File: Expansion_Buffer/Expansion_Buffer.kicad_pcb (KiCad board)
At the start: 2 copper layers, 23 x 62 mm, 18 parts, among them J1 Out, J2 In

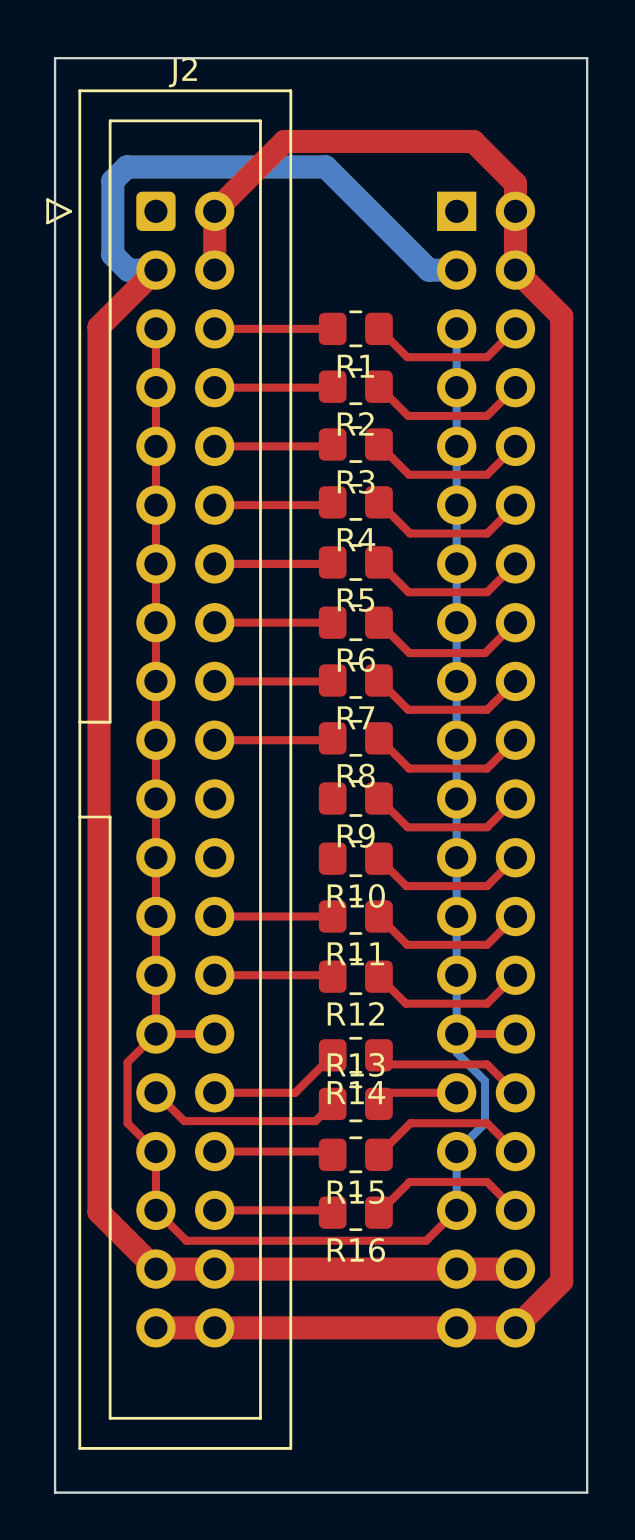
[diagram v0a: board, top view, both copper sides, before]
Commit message: added gerbers
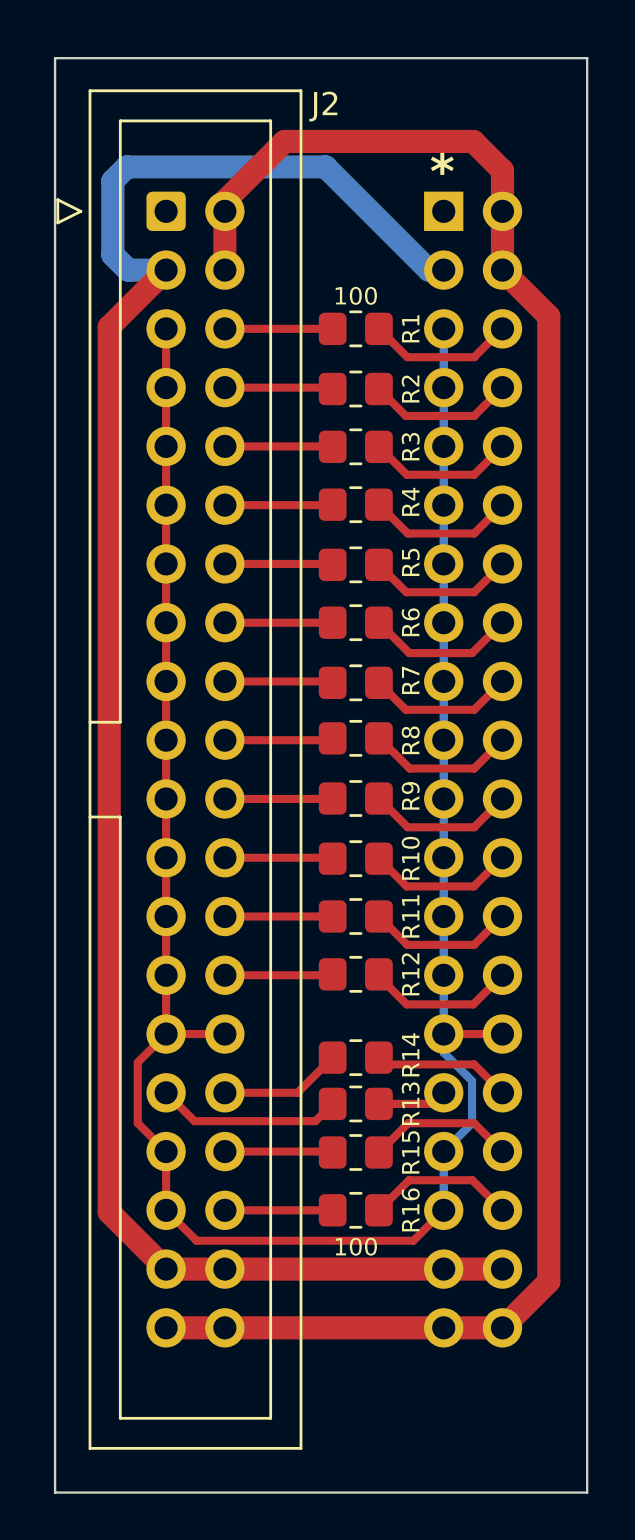
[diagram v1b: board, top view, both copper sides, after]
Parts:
- moved J1 0.56 mm to (108.8, 72.6)
- moved J2 0.44 mm to (96.8, 72.6)
- moved R12 0.10 mm to (105.0, 105.6)
- moved R14 0.10 mm to (105.0, 109.2)
- moved R15 0.10 mm to (105.0, 113.3)
- moved R16 0.10 mm to (105.0, 115.8)
- moved R5 0.10 mm to (105.0, 87.9)
- moved R2 0.10 mm to (105.0, 80.3)
- moved R3 0.10 mm to (105.0, 82.8)
- moved R4 0.10 mm to (105.0, 85.3)
- moved R7 0.10 mm to (105.0, 93.0)
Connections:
- J1 pad 10: Net-(J1-Pin_10) -> OUT3
- J1 pad 12: Net-(J1-Pin_12) -> OUT4
- J1 pad 14: Net-(J1-Pin_14) -> OUT5
- J1 pad 16: Net-(J1-Pin_16) -> OUT6
- J1 pad 18: Net-(J1-Pin_18) -> OUT7
- J1 pad 20: Net-(J1-Pin_20) -> OUT8
- J1 pad 22: Net-(J1-Pin_22) -> OUT9
- J1 pad 24: Net-(J1-Pin_24) -> OUT10
- J1 pad 26: Net-(J1-Pin_26) -> OUT11
- J1 pad 28: Net-(J1-Pin_28) -> OUT12
- J1 pad 31: Net-(J1-Pin_31) -> OUT13
- J1 pad 32: Net-(J1-Pin_32) -> OUT14
- J1 pad 34: Net-(J1-Pin_34) -> OUT15
- J1 pad 36: Net-(J1-Pin_36) -> OUT16
- J1 pad 6: Net-(J1-Pin_6) -> OUT1
- J1 pad 8: Net-(J1-Pin_8) -> OUT2
- J2 pad 10: OUT3 -> IN3
- J2 pad 12: OUT4 -> IN4
- J2 pad 14: OUT5 -> IN5
- J2 pad 16: OUT6 -> IN6
- J2 pad 18: OUT7 -> IN7
- J2 pad 20: OUT8 -> IN8
- J2 pad 22: OUT9 -> IN9
- J2 pad 24: OUT10 -> IN10
- J2 pad 26: OUT11 -> IN11
- J2 pad 28: OUT12 -> IN12
- J2 pad 31: OUT13 -> IN13
- J2 pad 32: OUT14 -> IN14
- J2 pad 34: OUT15 -> IN15
- J2 pad 36: OUT16 -> IN16
- J2 pad 6: OUT1 -> IN1
- J2 pad 8: OUT2 -> IN2
- R1 pad 1: Net-(J1-Pin_6) -> OUT1
- R1 pad 2: OUT1 -> IN1
- R10 pad 1: Net-(J1-Pin_24) -> OUT10
- R10 pad 2: OUT10 -> IN10
- R11 pad 1: Net-(J1-Pin_26) -> OUT11
- R11 pad 2: OUT11 -> IN11
- R12 pad 1: Net-(J1-Pin_28) -> OUT12
- R12 pad 2: OUT12 -> IN12
- R13 pad 1: OUT13 -> IN13
- R13 pad 2: Net-(J1-Pin_31) -> OUT13
- R14 pad 1: Net-(J1-Pin_32) -> OUT14
- R14 pad 2: OUT14 -> IN14
- R15 pad 1: Net-(J1-Pin_34) -> OUT15
- R15 pad 2: OUT15 -> IN15
- R16 pad 1: Net-(J1-Pin_36) -> OUT16
- R16 pad 2: OUT16 -> IN16
- R2 pad 1: Net-(J1-Pin_8) -> OUT2
- R2 pad 2: OUT2 -> IN2
- R3 pad 1: Net-(J1-Pin_10) -> OUT3
- R3 pad 2: OUT3 -> IN3
- R4 pad 1: Net-(J1-Pin_12) -> OUT4
- R4 pad 2: OUT4 -> IN4
- R5 pad 1: Net-(J1-Pin_14) -> OUT5
- R5 pad 2: OUT5 -> IN5
- R6 pad 1: Net-(J1-Pin_16) -> OUT6
- R6 pad 2: OUT6 -> IN6
- R7 pad 1: Net-(J1-Pin_18) -> OUT7
- R7 pad 2: OUT7 -> IN7
- R8 pad 1: Net-(J1-Pin_20) -> OUT8
- R8 pad 2: OUT8 -> IN8
- R9 pad 1: Net-(J1-Pin_22) -> OUT9
- R9 pad 2: OUT9 -> IN9
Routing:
- net IN13: track 0.00 -> 8.02 mm
- net Net-(J1-Pin_16): track 6.99 -> 0.00 mm
- net Net-(J1-Pin_34): track 6.97 -> 0.00 mm
- net Net-(J1-Pin_12): track 6.96 -> 0.00 mm
- net Net-(J1-Pin_36): track 6.96 -> 0.00 mm
- net Net-(J1-Pin_20): track 6.95 -> 0.00 mm
- net Net-(J1-Pin_10): track 6.95 -> 0.00 mm
- net Net-(J1-Pin_14): track 6.94 -> 0.00 mm
- net Net-(J1-Pin_8): track 6.93 -> 0.00 mm
- net Net-(J1-Pin_18): track 6.93 -> 0.00 mm
- net Net-(J1-Pin_22): track 6.92 -> 0.00 mm
- net Net-(J1-Pin_26): track 6.91 -> 0.00 mm
- net Net-(J1-Pin_6): track 6.91 -> 0.00 mm
- net Net-(J1-Pin_24): track 6.90 -> 0.00 mm
- net Net-(J1-Pin_28): track 6.89 -> 0.00 mm
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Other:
- board text added: "*"
